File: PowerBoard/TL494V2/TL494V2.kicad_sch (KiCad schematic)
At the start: 66 parts, among them J1 AuxConn, Q1 MMBTA92, Q2 CPC3980, Q5 IRFS4227TRLPBF, U1 TL494, U3 IR2181, U4 TL431

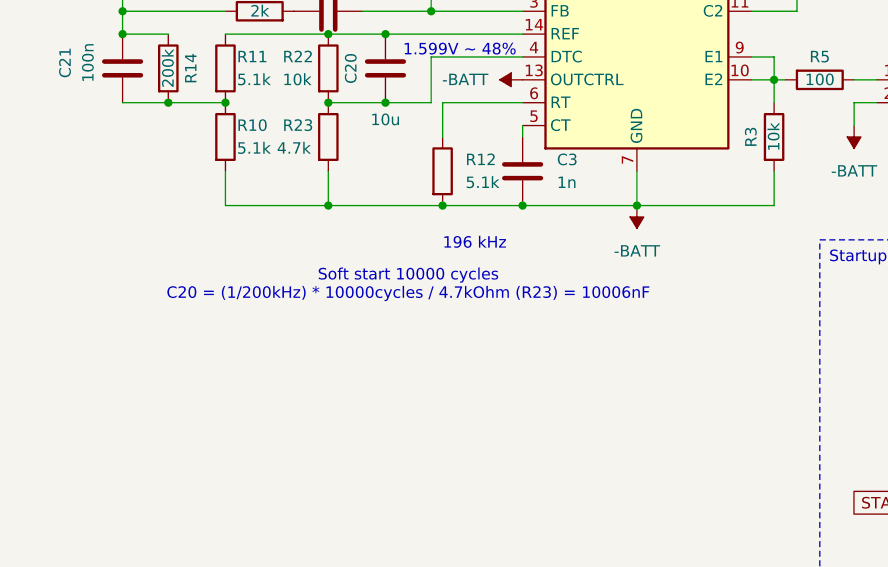
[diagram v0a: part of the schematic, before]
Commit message: cleanup
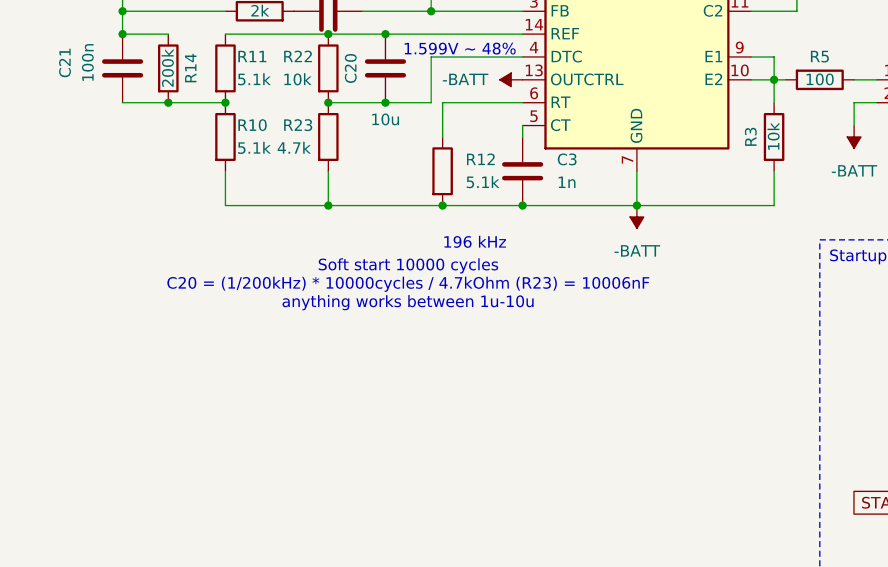
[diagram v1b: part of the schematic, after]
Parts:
- C20: MPN C14663 -> C96446
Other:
- note added: "Soft start 10000 cycles C20 = (1/200kHz) * 10000cycles / 4.7kOhm (R23) = 10006nF anything works between 1u-10u"
- note removed: "Soft start 10000 cycles C20 = (1/200kHz) * 10000cycles / 4.7kOhm (R23) = 10006nF"
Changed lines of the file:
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@@
 		)
 	)
-	(text "Soft start 10000 cycles\nC20 = (1/200kHz) * 10000cycles / 4.7kOhm (R23) = 10006nF\n"
+	(text "Soft start 10000 cycles\nC20 = (1/200kHz) * 10000cycles / 4.7kOhm (R23) = 10006nF\nanything works between 1u-10u"
 		(exclude_from_sim no)
 		(at 59.69 148.59 0)
@@
 			)
 		)
-		(property "MPN" "C14663"
+		(property "MPN" "C96446"
 			(at -10.16 101.6 90)
 			(effects
